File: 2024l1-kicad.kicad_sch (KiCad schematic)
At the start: 9 parts, among them IC1 SN74LVC2G04DRLR, IC2 SN74LVC2G04DRLR, J1 52610-1033, J2 XT60, J3 XT30, J4 XT30, J5 XT30, J6 XT30, J7 3V3_CONN

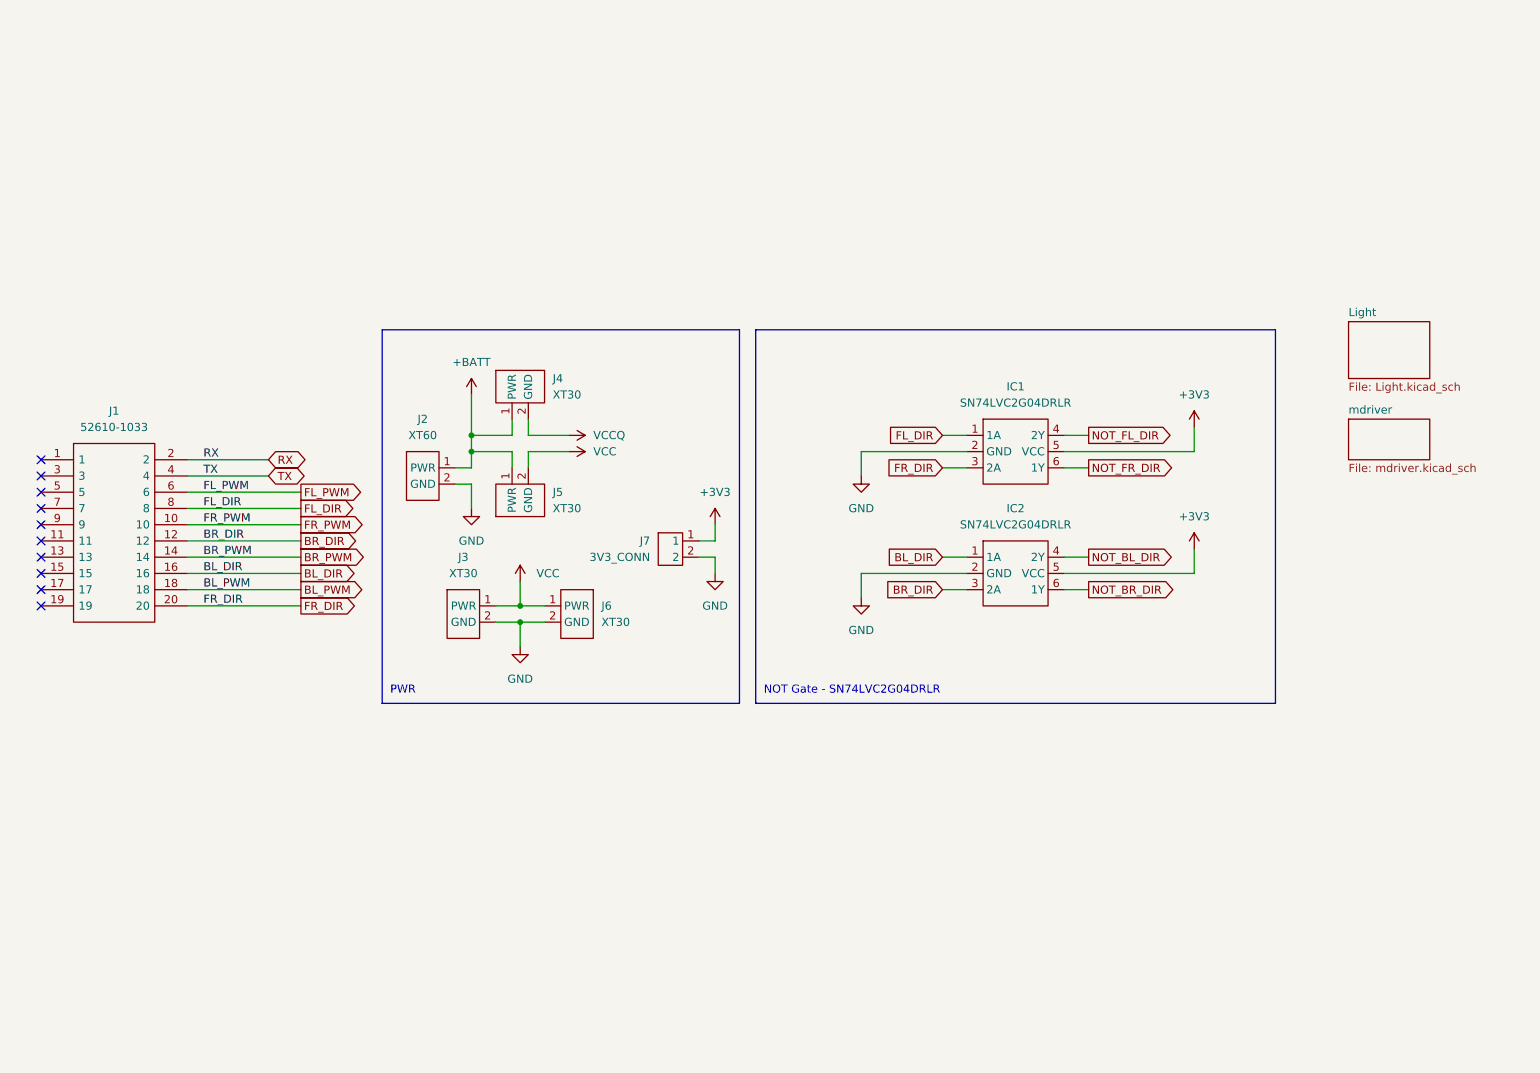
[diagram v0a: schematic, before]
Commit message: switches to stm32f0
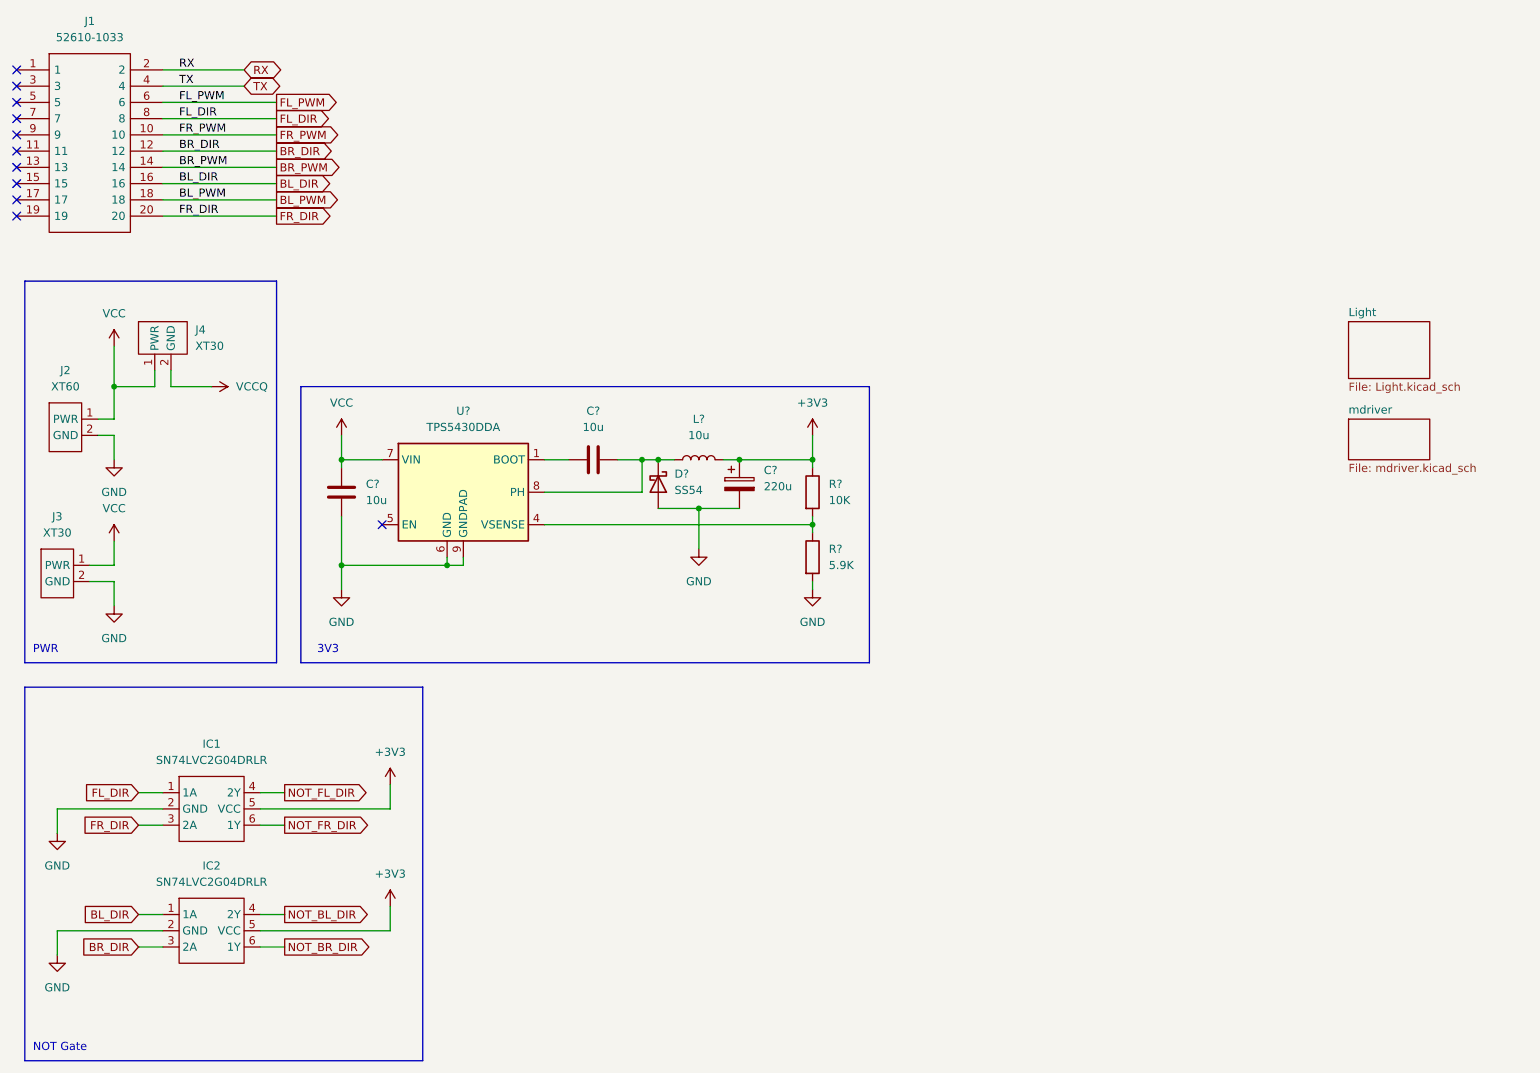
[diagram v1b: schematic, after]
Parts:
- removed J5, J6: XT30, symbol Connector_XT:XT30
- removed J7: 3V3_CONN, symbol Connector_JST:BM02B-SRSS-TB
- added C?: 220u, symbol Device:C_Polarized
- added C? (x2): 10u, symbol Device:C
- added D?: SS54, symbol Device:D_Schottky
- added L?: 10u, symbol Device:L
- added R?: 5.9K, symbol Device:R
- added R?: 10K, symbol Device:R
- added U?: TPS5430DDA, Package_SO:TI_SO-PowerPAD-8_ThermalVias, symbol Regulator_Switching:TPS5430DDA
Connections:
- net +BATT is gone; now on net VCC: J2.1 (PWR), J4.1 (PWR)
- net +3V3: now also C?.1, L?.2, R?.1
- net GND: now also C?.2, C?.2, D?.2 (A), R?.2, U?.6 (GND), U?.9 (GNDPAD)
- net VCC: now also C?.1, U?.7 (VIN)
- new net: C?.2, D?.1 (K), L?.1, U?.8 (PH)
- new net: R?.1, R?.2, U?.4 (VSENSE)
- new net: C?.1, U?.1 (BOOT)
- no-connect marks 10 -> 11
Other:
- note added: "3V3"
- note added: "NOT Gate"
- note removed: "NOT Gate - SN74LVC2G04DRLR"
- moved on the sheet: IC1, IC2, J1, J2, J3, J4
